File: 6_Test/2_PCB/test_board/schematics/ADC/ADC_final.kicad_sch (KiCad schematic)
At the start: 5 parts, among them J6 GND_AVSS_Connectors

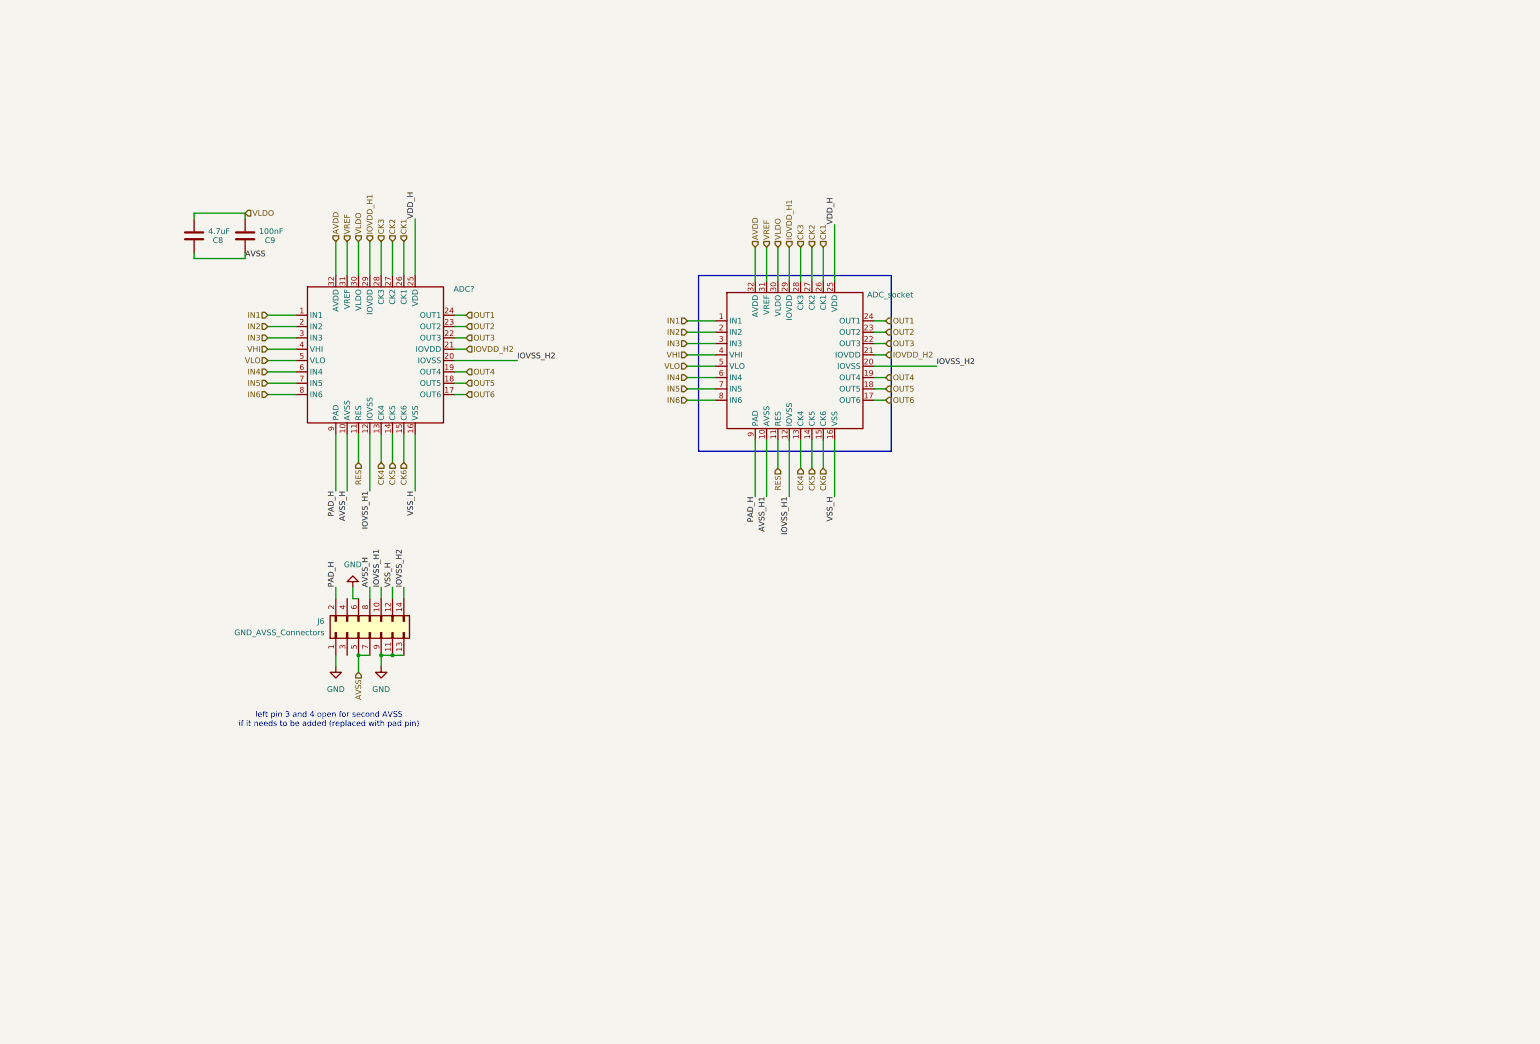
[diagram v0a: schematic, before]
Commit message: Adjusted Edits 11_25_24
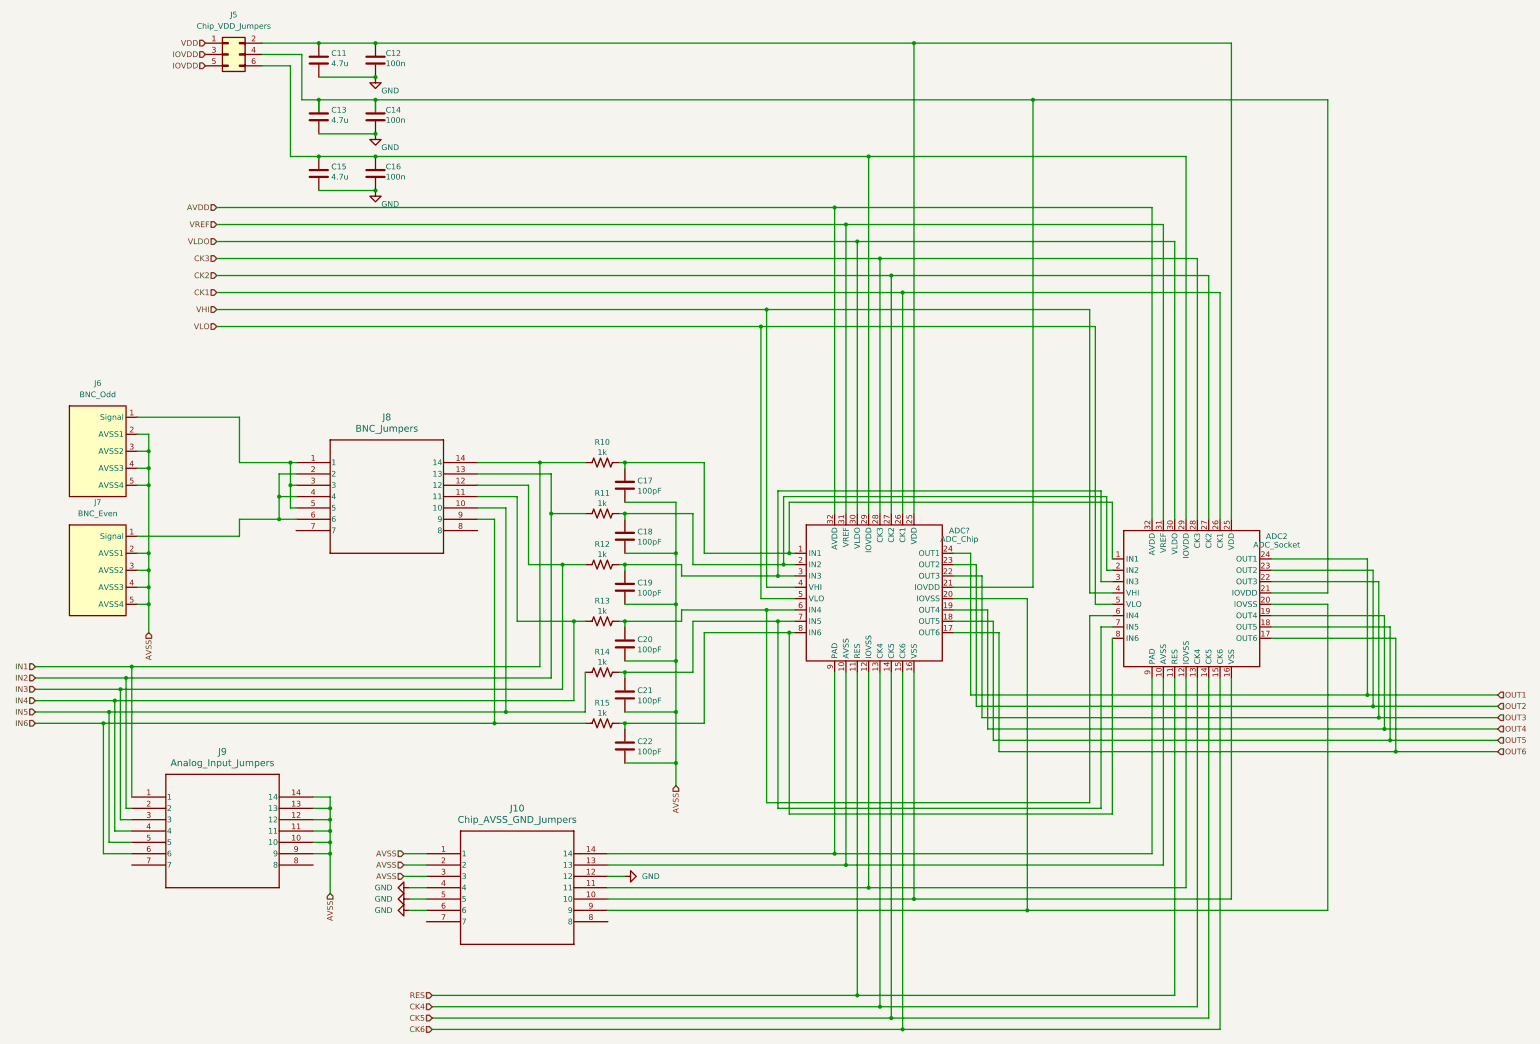
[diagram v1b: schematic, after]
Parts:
- removed C8: 4.7uF, Capacitor_SMD:C_0201_0603Metric, symbol Device:C
- removed C9: 100nF, Capacitor_SMD:C_0201_0603Metric, symbol Device:C
- removed J6: GND_AVSS_Connectors, Connector_PinHeader_2.54mm:PinHeader_2x07_P2.54mm_Vertical, symbol Connector_Generic:Conn_02x07_Odd_Even
- added C11, C13, C15: 4.7u, Capacitor_SMD:C_0603_1608Metric, symbol Device:C
- added C12, C14, C16: 100n, Capacitor_SMD:C_0402_1005Metric, symbol Device:C
- added C17, C18, C19, C20, C21, C22: 100pF, cap100pFFootprints:G-033_MUR, symbol Device:C
- added J10: Chip_AVSS_GND_Jumpers, ECE628_lib:6x2header, symbol 6x2Header:TSW-107-07-F-D
- added J5: Chip_VDD_Jumpers, Connector_PinHeader_2.54mm:PinHeader_2x03_P2.54mm_Vertical, symbol Connector_Generic:Conn_02x03_Odd_Even
- added J6: BNC_Odd, ECE628_lib:bnc_mini_gnd, symbol bnc_mini_gnd:bnc_mini_gnd
- added J7: BNC_Even, ECE628_lib:bnc_mini_gnd, symbol bnc_mini_gnd:bnc_mini_gnd
- added J8: BNC_Jumpers, TSW-107-07-G-D_SAI, symbol 6x2Header:TSW-107-07-F-D
- added J9: Analog_Input_Jumpers, TSW-107-07-G-D_SAI, symbol 6x2Header:TSW-107-07-F-D
- added R10, R11, R12, R13, R14, R15: 1k, symbol Device:R_US
- ADC2: renamed from ADC_socket; value ~ -> ADC_Socket; footprint Package_DFN_QFN:QFN-32-1EP_5x5mm_P0.5mm_EP3.1x3.1mm_ThermalVias -> Package_DIP:DIP-32_W15.24mm_Socket
- ADC?: value ~ -> ADC_Chip
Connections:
- net AVSS_H1 is gone; now on an unnamed net: ADC2.10 (AVSS)
- net AVSS: now also C17.2, C18.2, C19.2, C20.2, C21.2, C22.2, J10.1, J10.2, J10.3, J6.2 (AVSS1), J6.3 (AVSS2), J6.4 (AVSS3), J6.5 (AVSS4), J7.2 (AVSS1), J7.3 (AVSS2), J7.4 (AVSS3), J7.5 (AVSS4), J9.10, J9.11, J9.12, J9.13, J9.14, J9.9
- net GND: now also C11.2, C12.2, C13.2, C14.2, C15.2, C16.2, J10.12, J10.4, J10.5, J10.6
- net IN1: now also J8.14, J9.1, R10.1; no longer ADC2.1 (IN1), ADC?.1 (IN1)
- net IN2: now also J8.13, J9.2, R11.1; no longer ADC2.2 (IN2), ADC?.2 (IN2)
- net IN3: now also J8.12, J9.3, R12.1; no longer ADC2.3 (IN3), ADC?.3 (IN3)
- net IN4: now also J8.11, J9.4, R13.1; no longer ADC2.6 (IN4), ADC?.6 (IN4)
- net IN5: now also J8.10, J9.5, R14.1; no longer ADC2.7 (IN5), ADC?.7 (IN5)
- net IN6: now also J8.9, J9.6, R15.1; no longer ADC2.8 (IN6), ADC?.8 (IN6)
- net AVSS_H: no longer names the net of ADC?.10 (AVSS)
- net AVSS_H: now also J10.13
- net IOVDD_H1: no longer names the net of ADC2.29 (IOVDD), ADC?.29 (IOVDD)
- net IOVDD_H1: now also C15.1, C16.1, J5.6 (Pin_6)
- net IOVDD_H2: no longer names the net of ADC2.21 (IOVDD), ADC?.21 (IOVDD)
- net IOVDD_H2: now also C13.1, C14.1, J5.4 (Pin_4)
- net IOVSS_H1: no longer names the net of ADC2.12 (IOVSS), ADC?.12 (IOVSS)
- net IOVSS_H1: now also J10.11
- net IOVSS_H2: no longer names the net of ADC2.20 (IOVSS), ADC?.20 (IOVSS)
- net IOVSS_H2: now also J10.9
- net PAD_H: no longer names the net of ADC2.9 (PAD), ADC?.9 (PAD)
- net PAD_H: now also J10.14
- net VDD_H: no longer names the net of ADC2.25 (VDD), ADC?.25 (VDD)
- net VDD_H: now also C11.1, C12.1, J5.2 (Pin_2)
- net VSS_H: no longer names the net of ADC2.16 (VSS), ADC?.16 (VSS)
- net VSS_H: now also J10.10
- new net: J6.1 (Signal), J8.1, J8.3, J8.5
- new net: ADC2.7 (IN5), ADC?.7 (IN5), C21.1, R14.2
- new net: ADC2.2 (IN2), ADC?.2 (IN2), C18.1, R11.2
- new net: ADC2.6 (IN4), ADC?.6 (IN4), C20.1, R13.2
- new net: ADC2.8 (IN6), ADC?.8 (IN6), C22.1, R15.2
- new net: ADC2.1 (IN1), ADC?.1 (IN1), C17.1, R10.2
- new net: J7.1 (Signal), J8.2, J8.4, J8.6
- new net: ADC2.3 (IN3), ADC?.3 (IN3), C19.1, R12.2
- new net IOVDD: J5.3 (Pin_3), J5.5 (Pin_5)
- new net VDD: J5.1 (Pin_1)
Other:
- note removed: "left pin 3 and 4 open for second AVSS if it needs to be added (replaced with pad pin)"
- title: (none) -> ADC
- moved on the sheet: ADC2, ADC?
